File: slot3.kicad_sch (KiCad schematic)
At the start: 1 part

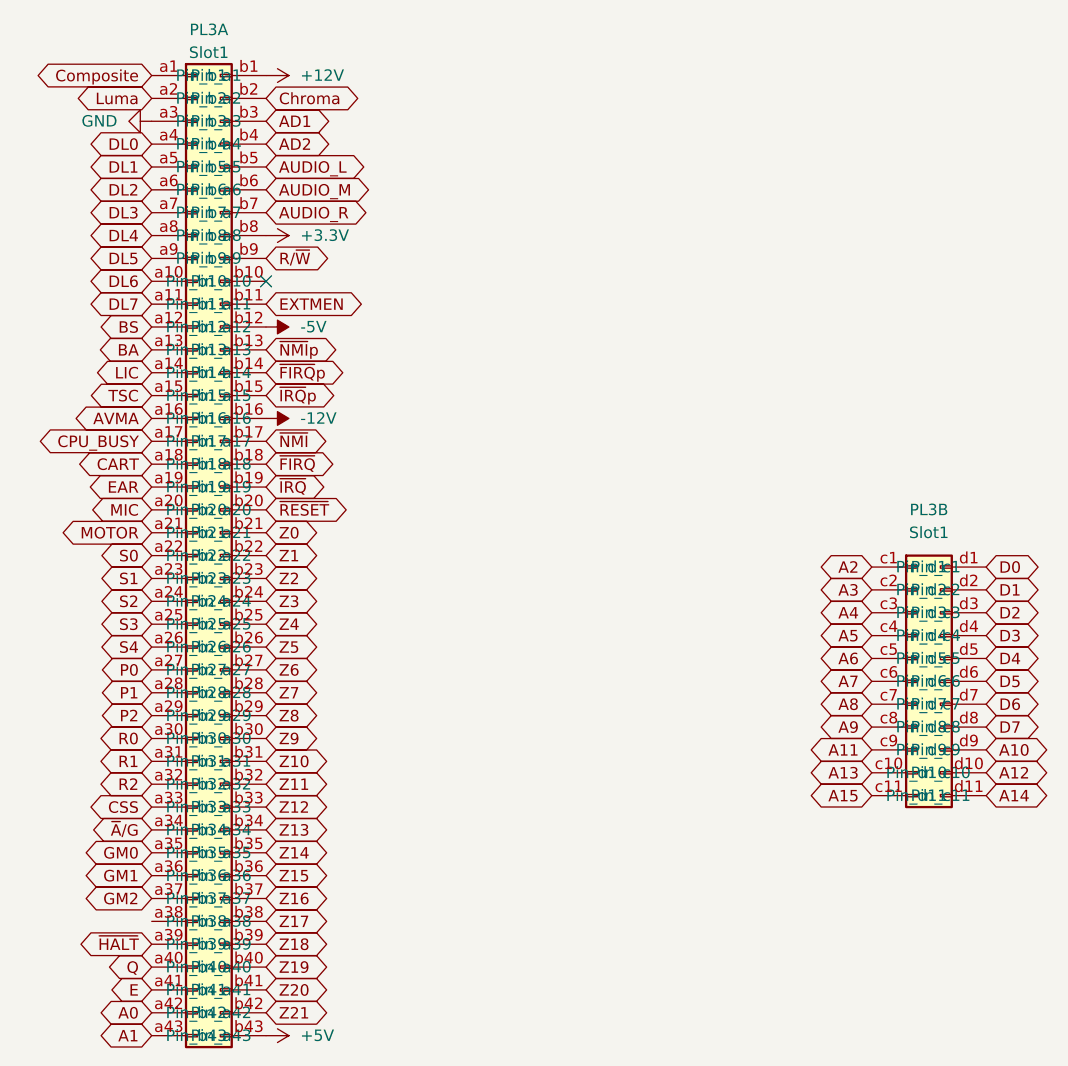
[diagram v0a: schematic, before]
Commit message: board layout
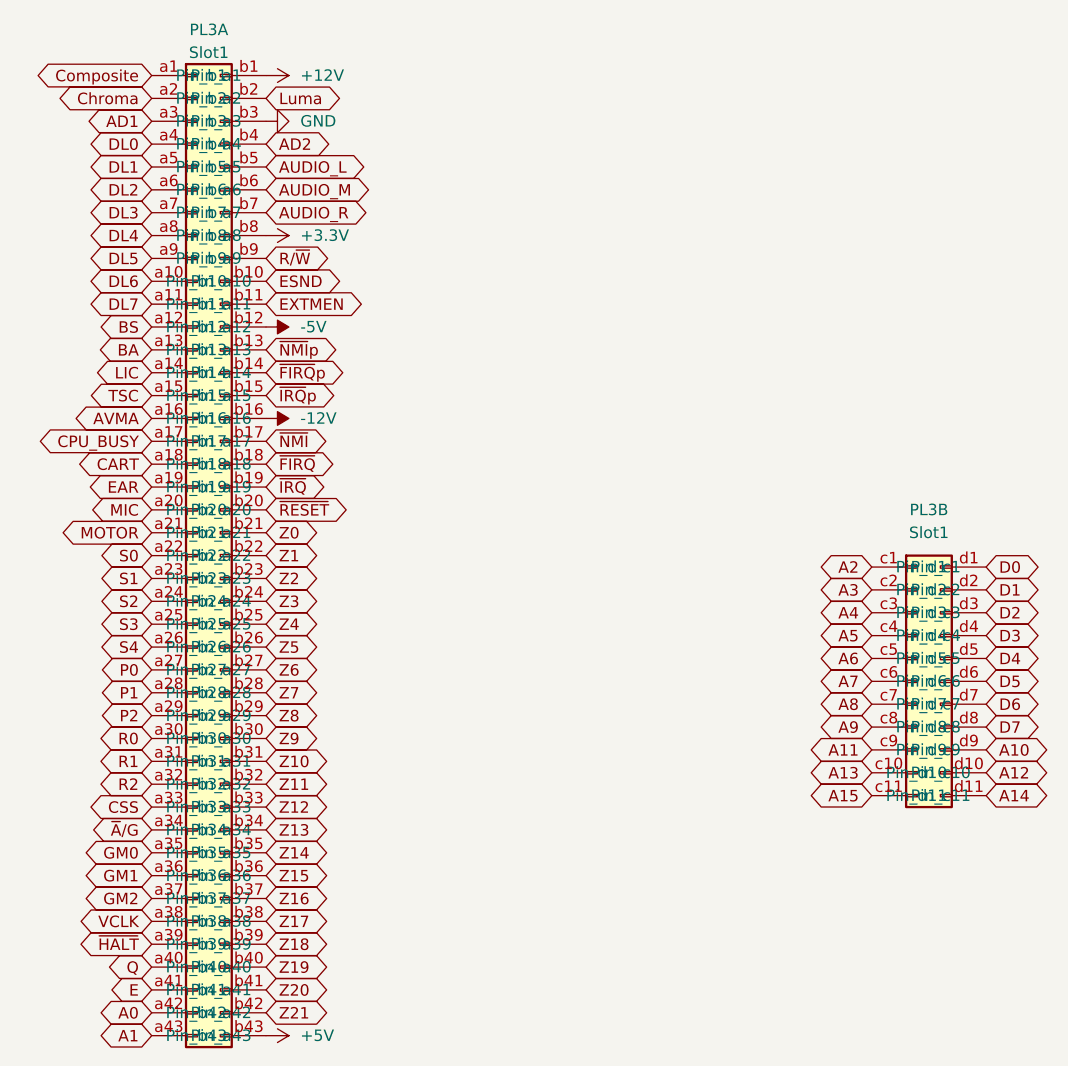
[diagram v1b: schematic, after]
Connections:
- net AD1: now also PL3.a3 (Pin_a3); no longer PL3.b3 (Pin_b3)
- net Chroma: now also PL3.a2 (Pin_a2); no longer PL3.b2 (Pin_b2)
- net GND: now also PL3.b3 (Pin_b3); no longer PL3.a3 (Pin_a3)
- net Luma: now also PL3.b2 (Pin_b2); no longer PL3.a2 (Pin_a2)
- net VCLK: now reaches PL3.a38 (Pin_a38)
- net ESND: now reaches PL3.b10 (Pin_b10)
- no-connect marks 1 -> 0
